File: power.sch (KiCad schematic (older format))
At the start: 23 parts, among them P1 CONN_01X02, P2 CONN_01X02, P23 CONN_01X02, P24 CONN_01X02, P3 CONN_01X02, P4 CONN_01X02, U1 ST1S14PHR

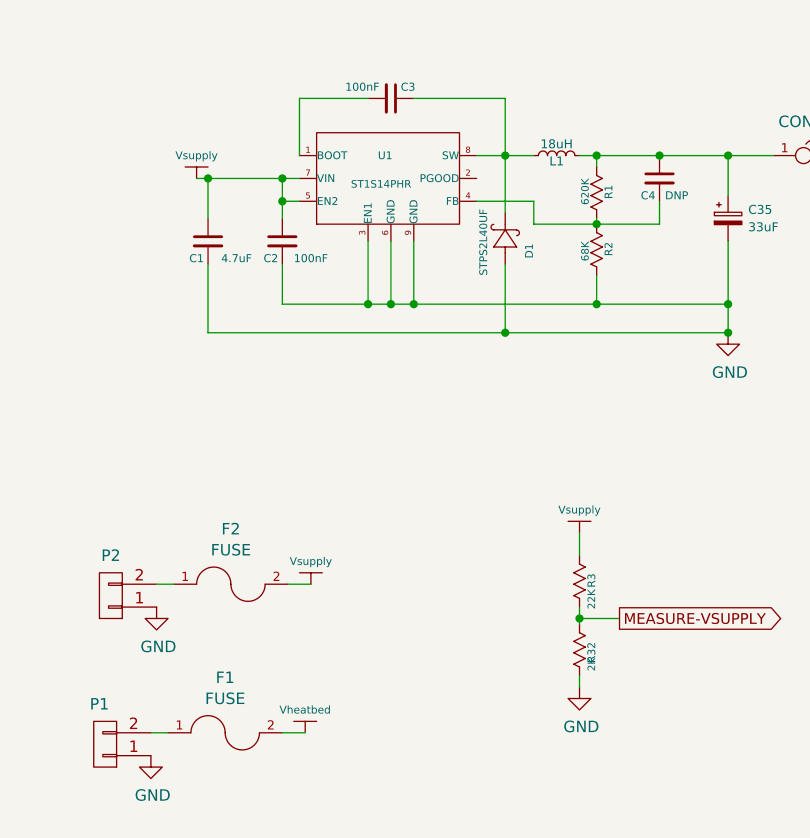
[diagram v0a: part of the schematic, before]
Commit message: More specs
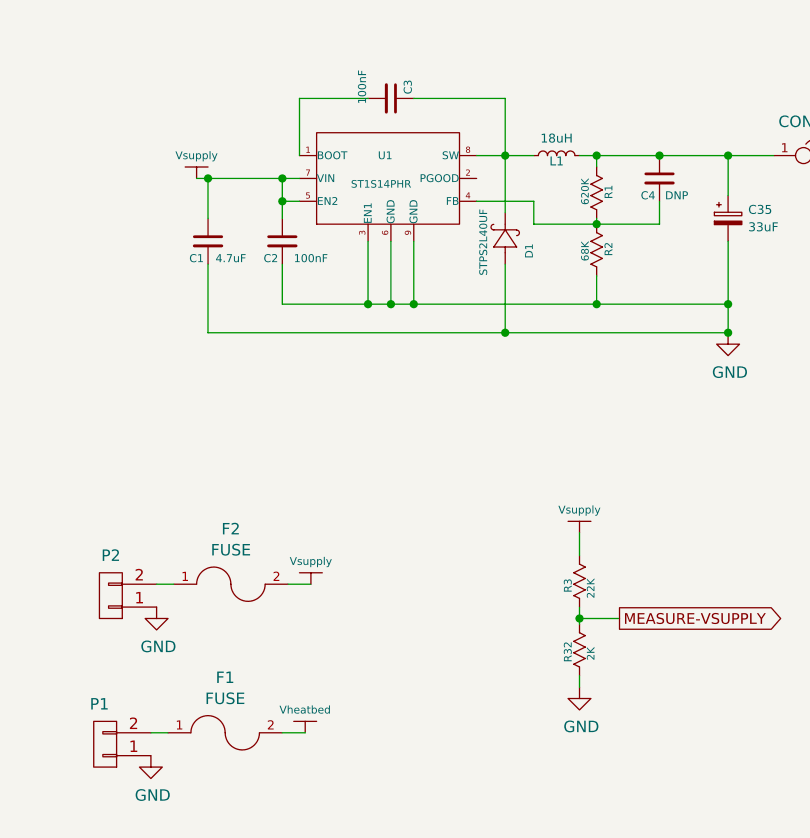
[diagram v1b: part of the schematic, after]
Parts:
- C1: VoltageRating (none) -> 50V
- C35: VoltageRating (none) -> 25V
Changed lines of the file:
@@
 U 1 1 56BDE999
 P 2475 1575
-F 0 "C3" V 2425 1650 35  0000 C CNN
-F 1 "100nF" V 2425 1450 35  0000 C CNN
+F 0 "C3" H 2425 1650 35  0000 C CNN
+F 1 "100nF" H 2425 1450 35  0000 C CNN
 F 2 "capacitors:C_0603" H 2475 1575 50  0001 C CNN
 F 3 "" H 2475 1575 50  0000 C CNN
@@
 F 4 "Panasonic" H 3950 2100 135 0001 L CNN "Manufacturer"
 F 5 "EEE-FK1E330W" H 3950 2100 135 0001 L CNN "ManufacturerNo"
+F 6 "25V" H 3950 2100 135 0001 L CNN "VoltageRating"
 	1    3950 2100
 	1    0    0    -1
@@
 P 1675 2200
 F 0 "C1" H 1625 2125 35  0000 C CNN
-F 1 "4.7uF" H 1800 2125 35  0000 C CNN
+F 1 "4.7uF" H 1775 2125 35  0000 C CNN
 F 2 "capacitors:C_1210" H 1675 2200 50  0001 C CNN
 F 3 "" H 1675 2200 50  0000 C CNN
 F 4 "Murata" H 1675 2200 135 0001 L CNN "Manufacturer"
 F 5 "GRM32ER71H475KA88L" H 1675 2200 135 0001 L CNN "ManufacturerNo"
+F 6 "50V" H 1675 2200 135 0001 L CNN "VoltageRating"
 	1    1675 2200
 	1    0    0    -1
@@
 P 3200 1825
 F 0 "L1" V 3175 1825 39  0000 C CNN
-F 1 "18uH" V 3250 1825 39  0000 C CNN
+F 1 "18uH" V 3275 1825 39  0000 C CNN
 F 2 "inductors:INDUCTOR_BOURNS_RLB914" H 3294 1825 50  0001 C CNN
 F 3 "" H 3200 1825 50  0000 C CNN
@@
 U 1 1 56C4E772
 P 3225 3575
-F 0 "R3" H 3303 3703 34  0000 L CNN
-F 1 "22K" H 3372 3703 33  0000 L CNN
+F 0 "R3" H 3325 3600 34  0000 L CNN
+F 1 "22K" H 3325 3700 33  0000 L CNN
 F 2 "resistors:R_0603" H 3225 3575 60  0001 C CNN
 F 3 "" H 3225 3575 60  0000 C CNN
@@
 U 1 1 56C4E7F8
 P 3225 3875
-F 0 "R32" H 3303 4003 34  0000 L CNN
-F 1 "2K" H 3372 4003 33  0000 L CNN
+F 0 "R32" H 3300 3900 34  0000 L CNN
+F 1 "2K" H 3325 4000 33  0000 L CNN
 F 2 "resistors:R_0603" H 3225 3875 60  0001 C CNN
 F 3 "" H 3225 3875 60  0000 C CNN
